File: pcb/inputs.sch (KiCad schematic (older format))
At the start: 61 parts, among them U11 MPXA6115AC6U, U4 MAX9926UAEE+, U6 MPX4250AP

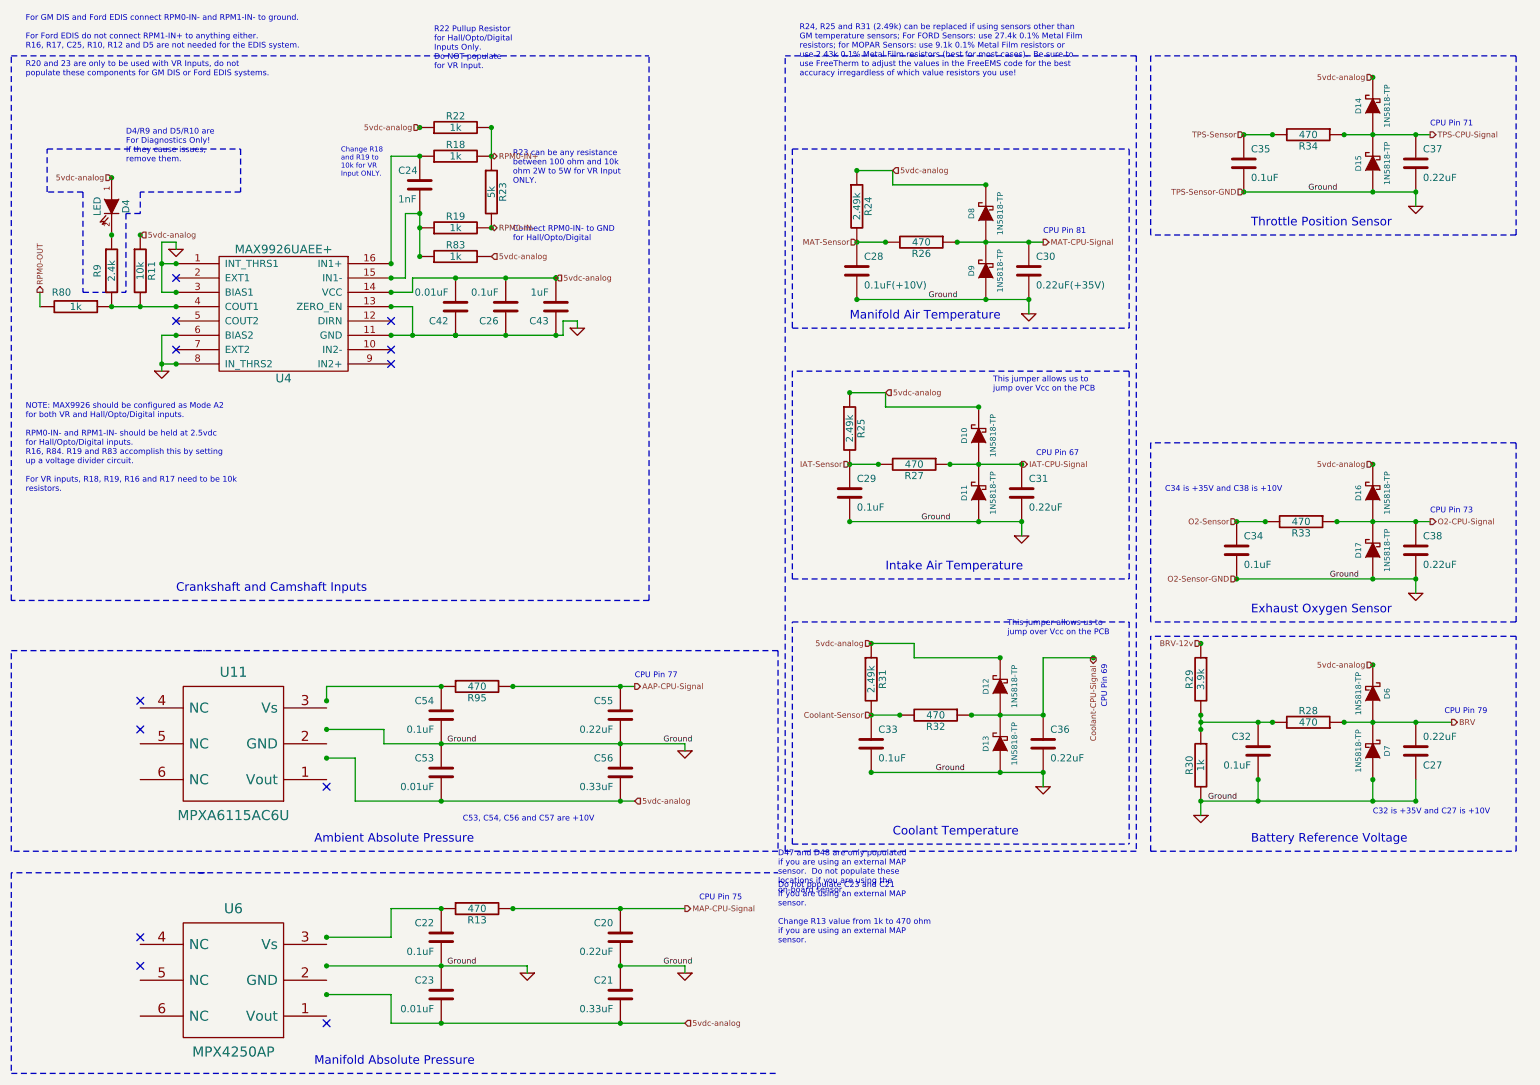
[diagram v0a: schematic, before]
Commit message: update
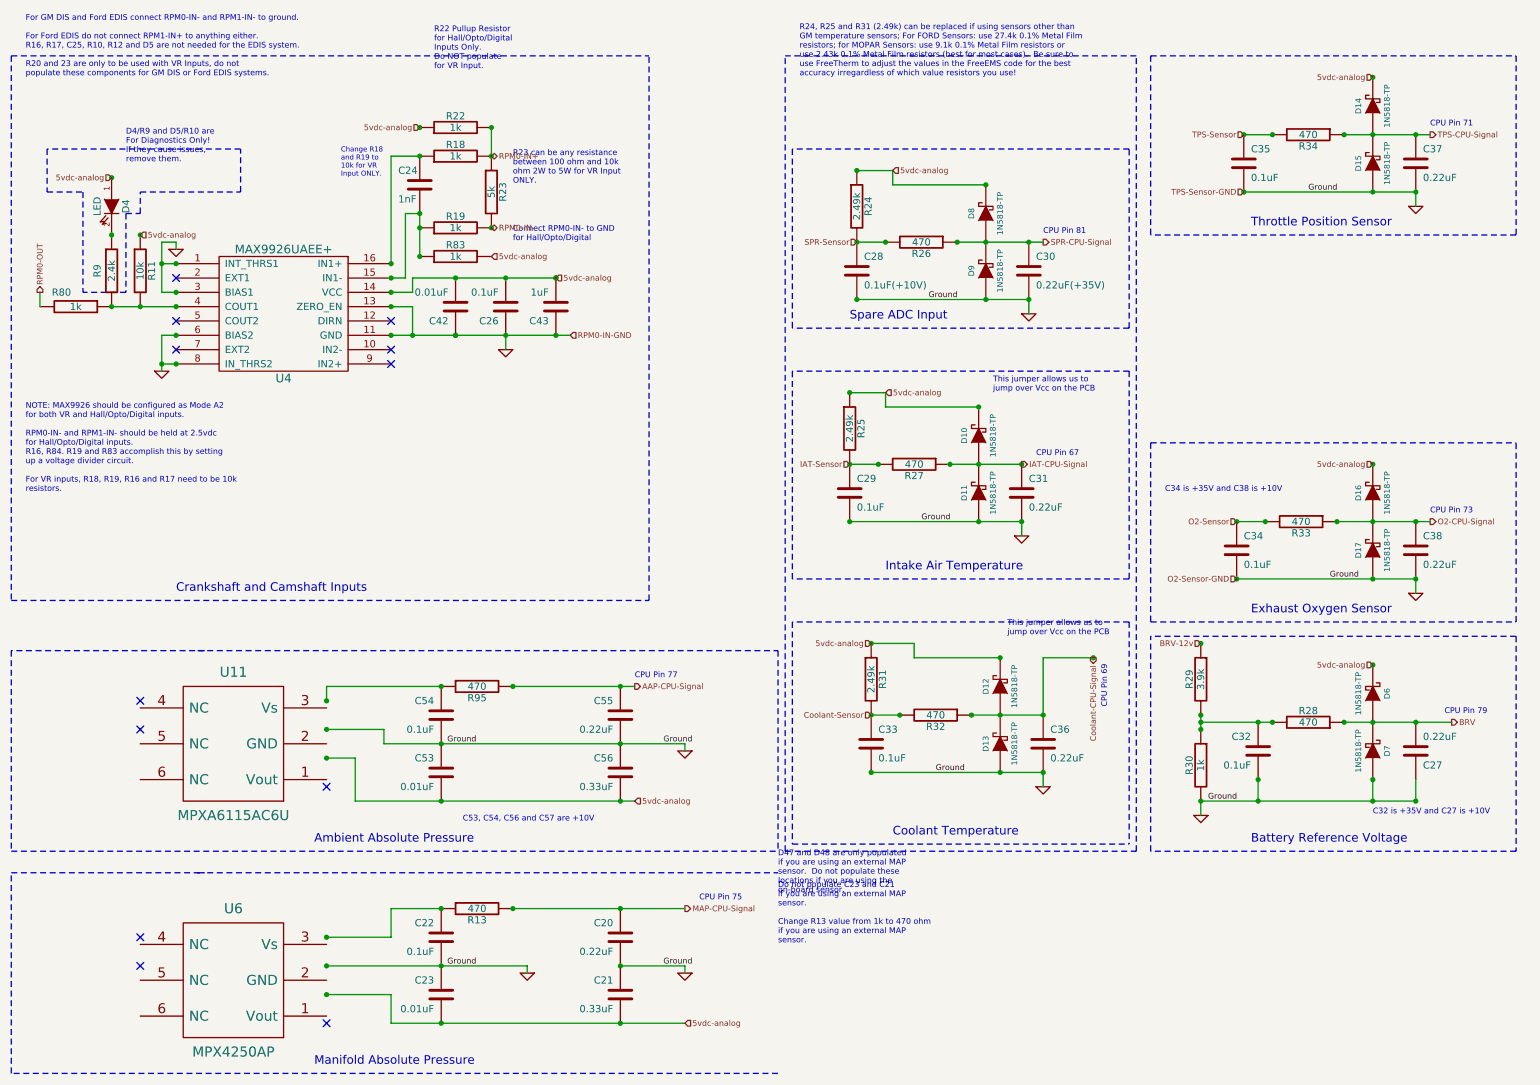
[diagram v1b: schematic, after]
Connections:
- net MAT-CPU-Signal renamed SPR-CPU-Signal
- net MAT-Sensor renamed SPR-Sensor
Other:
- note added: "Spare ADC Input"
- note removed: "Manifold Air Temperature"
